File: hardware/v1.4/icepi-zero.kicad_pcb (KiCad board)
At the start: 4 copper layers, 65 x 30 mm, 164 parts, among them J1 Conn_02x20_Counter_Clockwise, J2 GPDI_C_1.3, J3 USB_C_Receptacle_USB2.0_14P, J4 USB_C_Receptacle_USB2.0_14P, J5 USB_C_Receptacle_USB2.0_14P, J6 Micro_SD_Card_Det2, SW1 SW_Push, SW2 SW_Push, U1 ECP5-CABGA256, U10 TPD2EUSB30A, U11 W9825G6KH, U12 W25Q128JVS, U2 TLV62569DBV, U3 TLV62569DBV, U4 TLV62569DBV, U5 TPD2EUSB30A, U6 PCA9306DC1, U7 TPD2EUSB30A, U8 TPD2EUSB30A, U9 FT231XQ, Y1 SG-8018CG 50.000000MHz

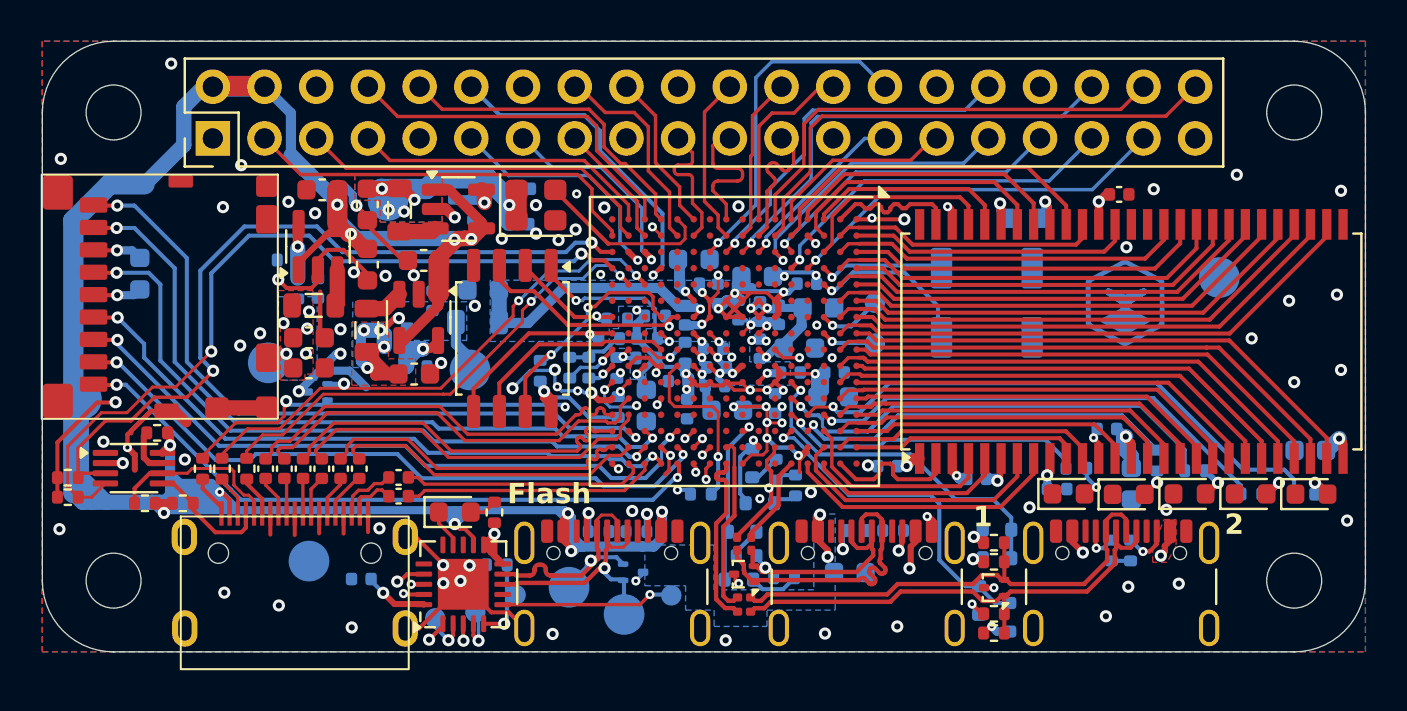
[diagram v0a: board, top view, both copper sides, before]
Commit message: Commit preliminary version of v1.4
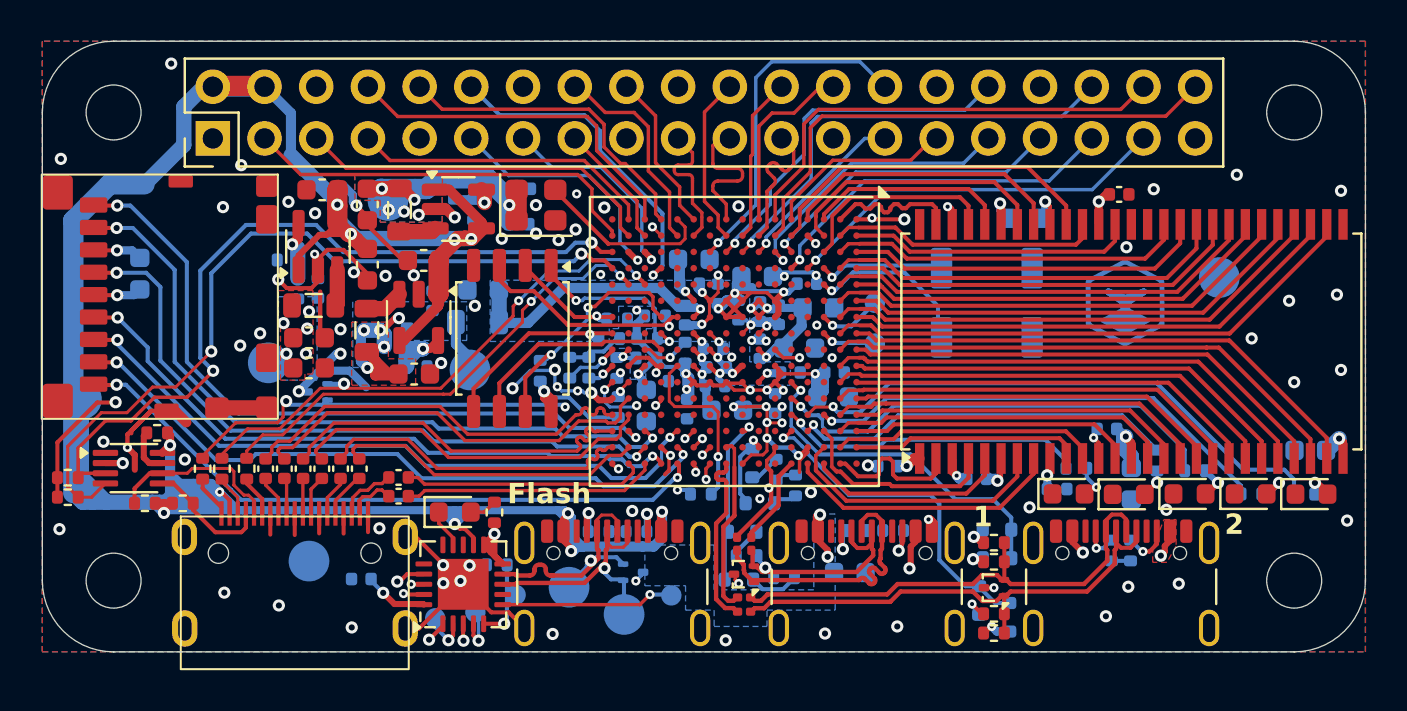
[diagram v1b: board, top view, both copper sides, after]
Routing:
- net GND: track 101.4 -> 102.2 mm, vias 109 -> 111

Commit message: Consolidated v1.4 version
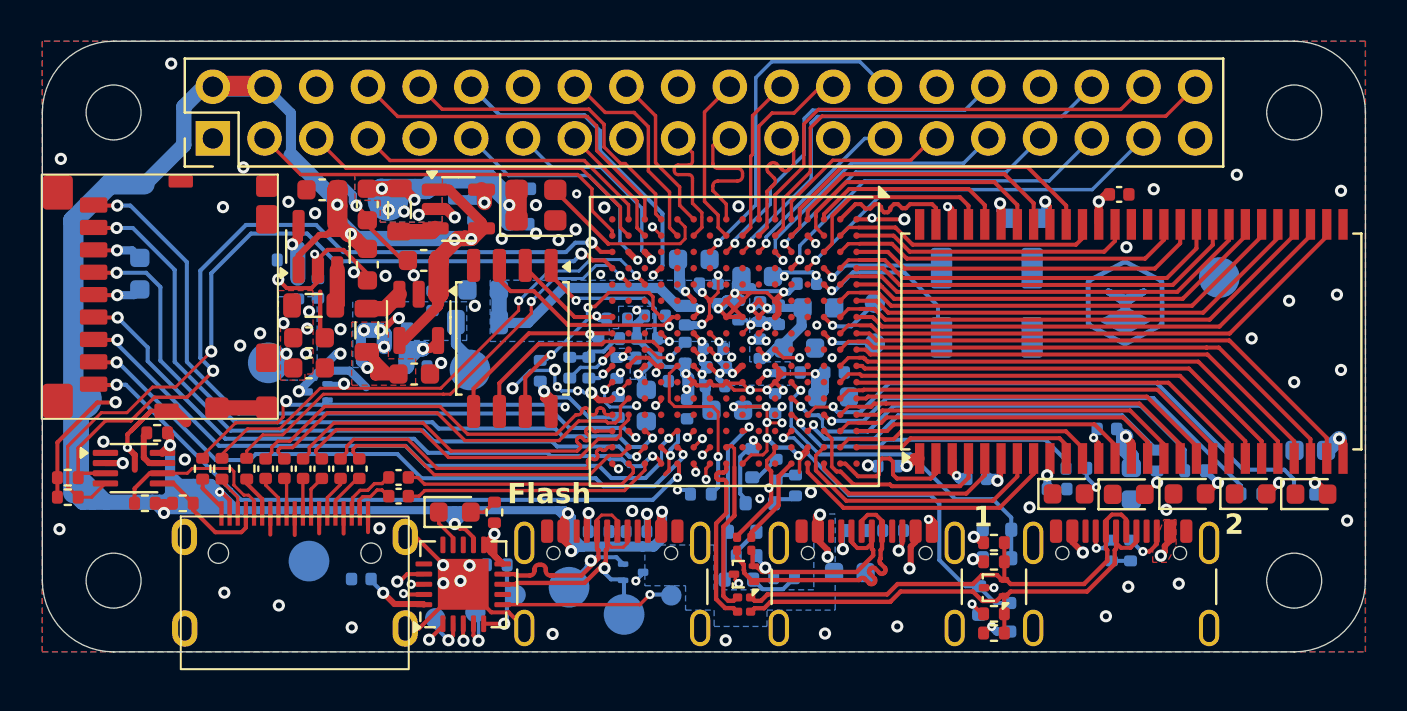
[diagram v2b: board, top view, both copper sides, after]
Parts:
- R48: value 15k -> 4.7k
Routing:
- net +3V3: track 93.9 -> 91.9 mm
- net GND: track 102.2 -> 103.4 mm
